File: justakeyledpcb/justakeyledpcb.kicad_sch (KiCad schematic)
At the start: 15 parts, among them SW1 SW_Push, SW2 SW_Push, SW3 SW_Push, SW4 SW_Push, U1 XIAO-RP2040-DIP

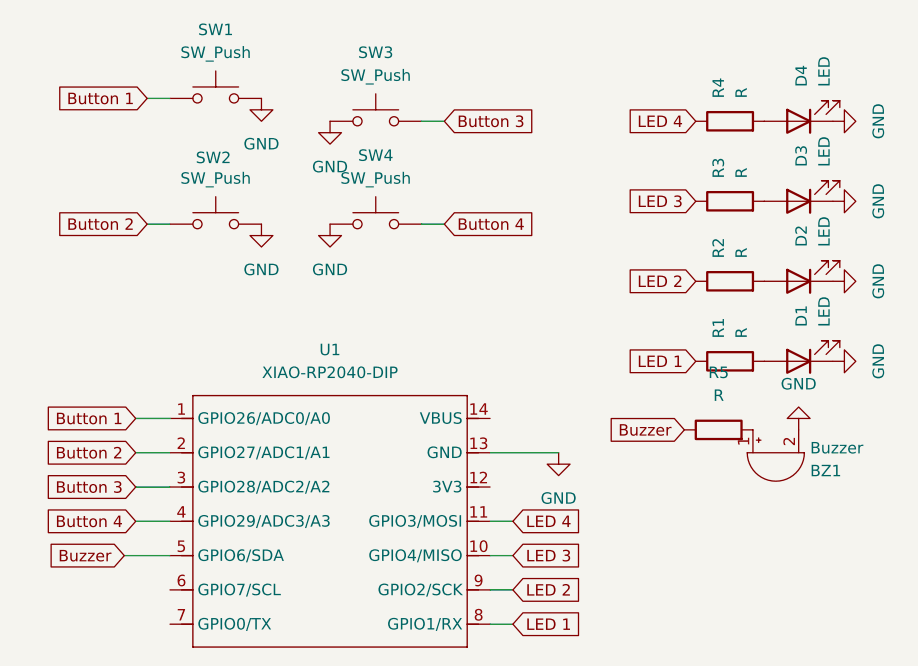
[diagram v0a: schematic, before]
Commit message: FInalised the PCB Schematics and PCB Layout
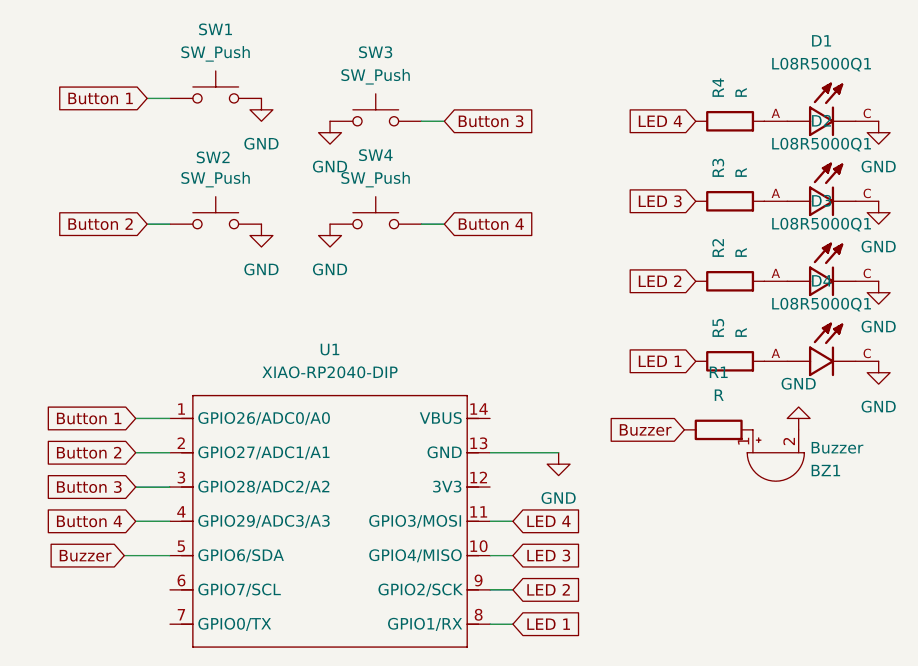
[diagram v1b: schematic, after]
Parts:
- removed D1, D2, D3, D4: LED, footprints:LEDRD254W57D500H1070, symbol Device:LED
- added D1, D2, D3, D4: L08R5000Q1, e390cee6c564169ed6d49fe7a268946ec8897500_l08r5000q1:LEDRD254W57D500H1070, symbol L08R5000Q1:L08R5000Q1
- renumbered R5 to R1, R1 to R5
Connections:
- net GND: now also D1.C, D2.C, D3.C, D4.C
- net at R2.2: now also D3.A
- net at R5.2: now also D4.A
- net at R4.2: now also D1.A
- net at R3.2: now also D2.A
